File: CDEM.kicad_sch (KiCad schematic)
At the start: 41 parts, among them J1 USB_C_Receptacle_USB2.0, J2 6P6C, J3 Conn_01x04, Q1 2N7002, Q2 S8050, Q3 S8050, SW1 BTN, SW2 RESET, U1 AMS1117-3.3, U2 USBLC6-2SC6, U3 CP2104, U4 ESP-12E

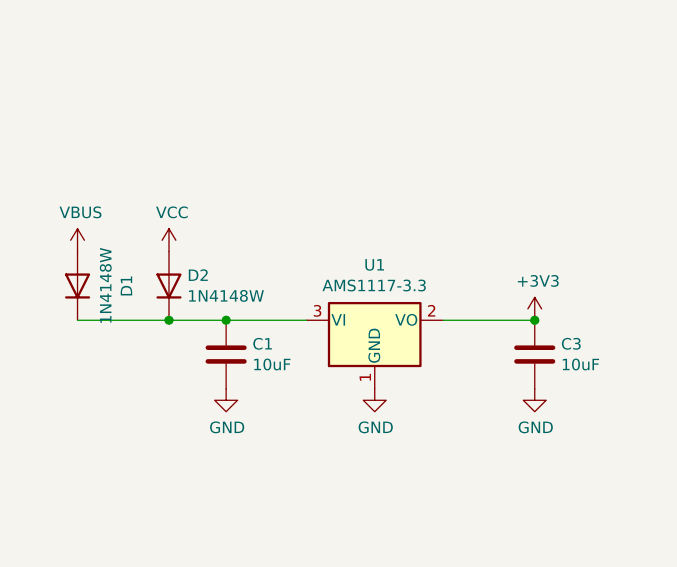
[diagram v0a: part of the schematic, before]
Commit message: fix power problem
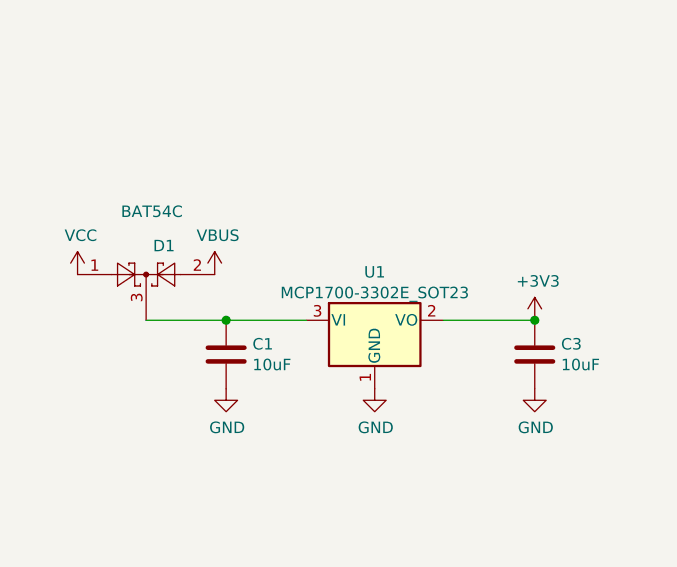
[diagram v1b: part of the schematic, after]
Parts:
- removed D1, D2: 1N4148W, Diode_SMD:D_SOD-123, symbol Diode:1N4148W
- removed U1: AMS1117-3.3, Package_TO_SOT_SMD:SOT-223-3_TabPin2, symbol Regulator_Linear:AMS1117-3.3
- added D1: BAT54C, Package_TO_SOT_SMD:SOT-23, symbol Diode:BAT54C
- added U1: MCP1700-3302E_SOT23, Package_TO_SOT_SMD:SOT-23, symbol Regulator_Linear:MCP1700-3302E_SOT23
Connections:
- net +3V3: now also U1.2 (VO)
- net GND: now also U1.1 (GND)
- net VBUS: now also D1.2
- net VCC: now also D1.1
- net at C1.1: now also D1.3, U1.3 (VI)
